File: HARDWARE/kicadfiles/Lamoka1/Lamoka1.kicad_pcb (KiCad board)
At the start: 2 copper layers, 33 parts

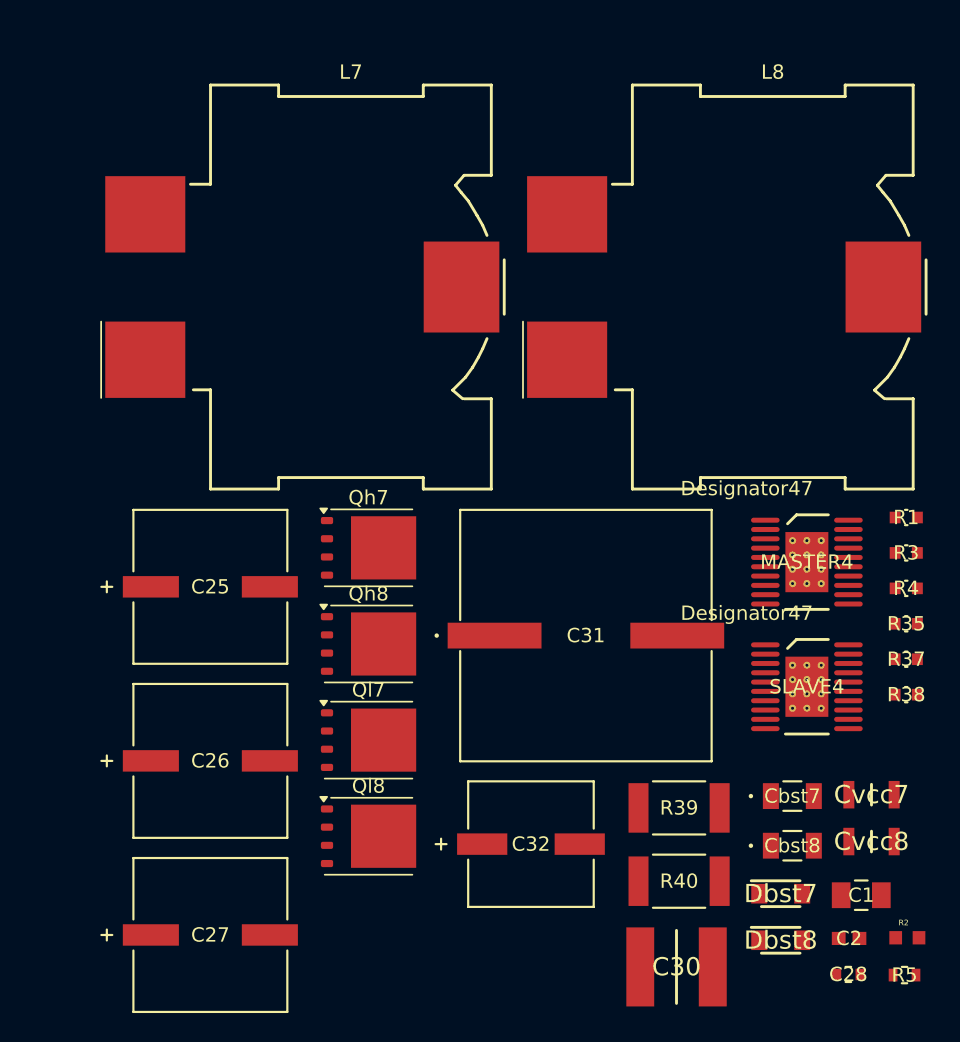
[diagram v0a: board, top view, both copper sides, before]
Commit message: Improve on the values for the schematic of boost converter
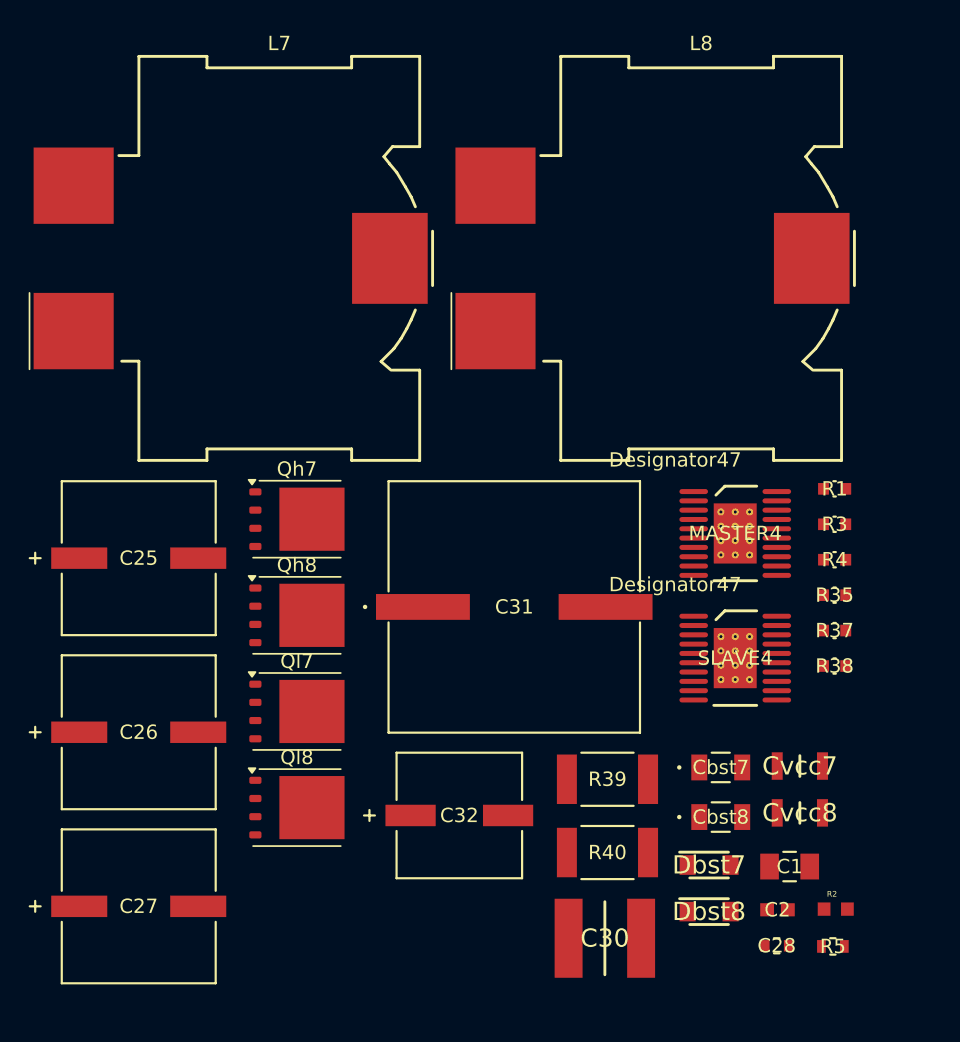
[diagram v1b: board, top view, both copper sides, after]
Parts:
- C1: value C1206C474K5RACTU -> 0.47u
- C2: value CC0603KRX7R9BB223 -> 22n
- C25, C26: value UUX2A470MNL1GS -> 47u
- C27, C32: value UCD2A220MNL1GS -> 22u
- C28: value CL10B104KB8NNNC -> 100n
- C30: value KRM55WR72A226MH01L -> 22u
- C31: value UCD2A101MNJ1MS -> 10u
- Cbst7: value C1206C224M1REC7210 -> 220n
- Cbst8: value C1206C224M1REC7210 -> 0.22u
- Cvcc7: value CNC5L1X7R1H106K160AE -> 100n
- Cvcc8: value CNC5L1X7R1H106K160AE -> 10u
- R1: value RC0603FR-0756K2L -> 56.2k
- R2: value RN73R1JTTD1842F25 -> 18.4k
- R3: value RC0603FR-07392KL -> 392k
- R35, R37, R38: value RC0603FR-0736KL -> 36k
- R39, R40: value TLRP3A30CR005FTE -> 5m
- R4: value RC0603FR-0710KL -> 10k
- R5: value RN73R1JTTD4992F25 -> 49.9k
- moved C25 5.39 mm to (125.7, 106.8)
- moved C26 5.39 mm to (125.7, 118.9)
- moved C27 5.39 mm to (125.7, 131.1)
- moved R40 5.39 mm to (158.4, 127.3)
- moved C1 5.39 mm to (171.1, 128.3)
- moved C2 5.39 mm to (170.3, 131.3)
- moved C28 5.39 mm to (170.2, 133.8)
- moved C30 5.39 mm to (158.2, 133.3)
- moved C31 5.39 mm to (151.9, 110.2)
- moved C32 5.39 mm to (148.1, 124.7)
- moved Cbst7 5.39 mm to (166.3, 121.4)
- moved Cbst8 5.39 mm to (166.3, 124.8)
- moved Cvcc7 5.39 mm to (171.8, 121.3)
- moved Cvcc8 5.39 mm to (171.8, 124.6)
- moved Dbst7 5.39 mm to (165.5, 128.2)
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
